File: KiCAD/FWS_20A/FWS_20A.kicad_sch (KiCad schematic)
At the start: 14 parts, among them J1 sense, J2 pwr, Q2 BC846, U1 XMSM0L1306SRGER, U2 FDMS8333L, U3 FDMS8333L, U4 LM5109BSD, U6 L78L33_SO8

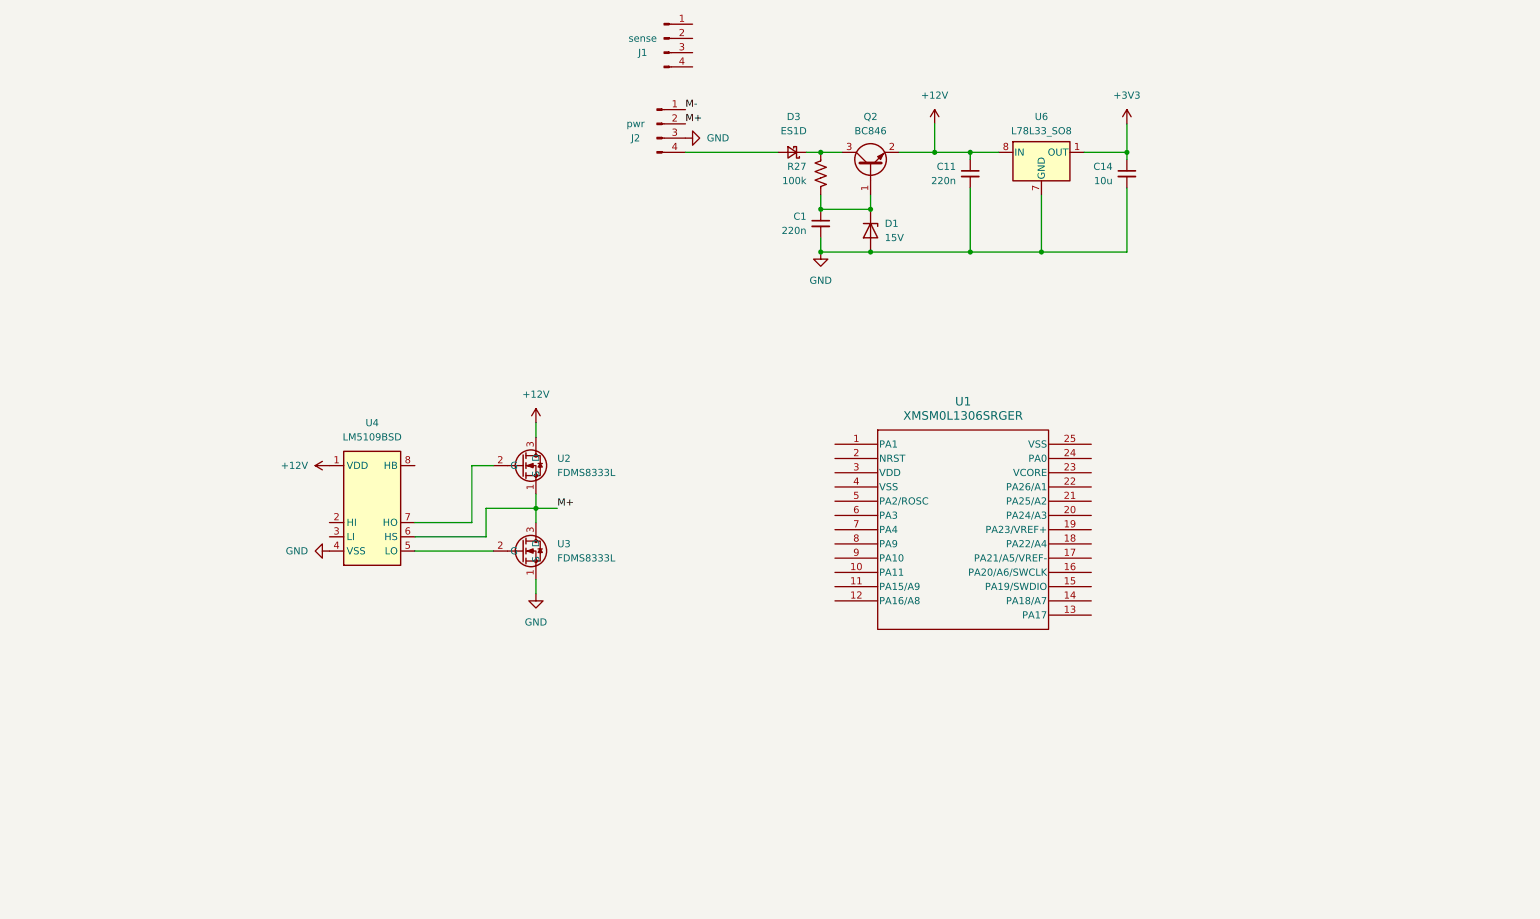
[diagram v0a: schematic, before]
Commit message: maybe schematic
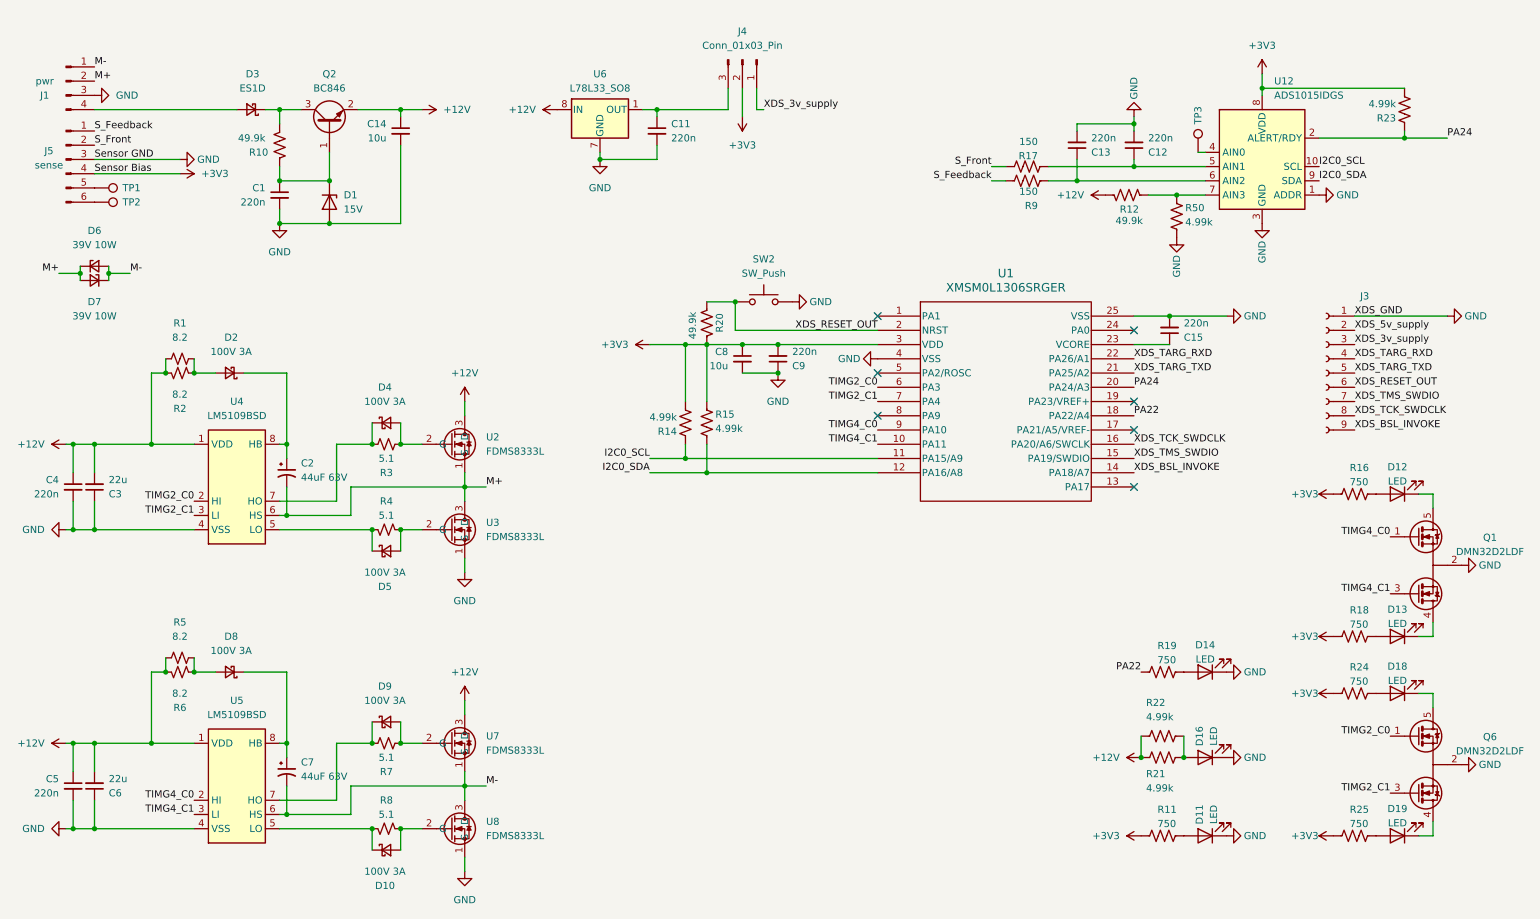
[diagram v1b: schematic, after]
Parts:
- removed J2: pwr, symbol Connector:Conn_01x04_Pin
- removed R27: 100k, Resistor_SMD:R_1206_3216Metric_Pad1.30x1.75mm_HandSolder, symbol Device:R_US
- added C12, C13, C15, C4, C5, C9: 220n, Capacitor_SMD:C_1206_3216Metric_Pad1.33x1.80mm_HandSolder, symbol Device:C_Small
- added C2, C7: 44uF 63V, Capacitor_THT:C_Radial_D6.3mm_H11.0mm_P2.50mm, symbol Device:C_Polarized_Small_US
- added C3, C6: 22u, Capacitor_SMD:C_1206_3216Metric_Pad1.33x1.80mm_HandSolder, symbol Device:C_Small
- added C8: 10u, Capacitor_SMD:C_1206_3216Metric_Pad1.33x1.80mm_HandSolder, symbol Device:C_Small
- added D10, D2, D4, D5, D8, D9: 100V 3A, FWS_footprints:PMDE, symbol Device:D_Schottky_Small
- added D11, D12, D13, D14, D16, D18, D19: LED, LED_SMD:LED_0603_1608Metric, symbol Device:LED
- added D6, D7: 39V 10W, Diode_SMD:D_SMC_Handsoldering, symbol Device:D_Zener_Small
- added J3: Conn_01x09_Socket, Connector_PinHeader_2.54mm:PinHeader_1x09_P2.54mm_Vertical, symbol Connector:Conn_01x09_Socket
- added J4: Conn_01x03_Pin, Connector_PinHeader_2.54mm:PinHeader_1x03_P2.54mm_Vertical, symbol Connector:Conn_01x03_Pin
- added J5: sense, Connector_Molex:Molex_Micro-Fit_3.0_43045-0600_2x03_P3.00mm_Horizontal, symbol Connector:Conn_01x06_Pin
- added Q1, Q6: DMN32D2LDF, Package_TO_SOT_SMD:SOT-353_SC-70-5, symbol Transistor_FET:DMN32D2LDF
- added R1, R2, R5, R6: 8.2, Resistor_SMD:R_2816_7142Metric_Pad3.20x4.45mm_HandSolder, symbol Device:R_Small_US
- added R10, R12, R20: 49.9k, Resistor_SMD:R_1206_3216Metric_Pad1.30x1.75mm_HandSolder, symbol Device:R_US
- added R11, R16, R18, R19, R24, R25: 750, Resistor_SMD:R_1206_3216Metric_Pad1.30x1.75mm_HandSolder, symbol Device:R_US
- added R14, R15, R21, R22, R23, R50: 4.99k, Resistor_SMD:R_1206_3216Metric_Pad1.30x1.75mm_HandSolder, symbol Device:R_US
- added R17, R9: 150, Resistor_SMD:R_1206_3216Metric_Pad1.30x1.75mm_HandSolder, symbol Device:R_US
- added R3, R4, R7, R8: 5.1, Resistor_SMD:R_2512_6332Metric_Pad1.40x3.35mm_HandSolder, symbol Device:R_Small_US
- added SW2: SW_Push, Button_Switch_SMD:SW_SPST_PTS645Sx43SMTR92, symbol Switch:SW_Push
- added TP1, TP2, TP3: TestPoint, TestPoint:TestPoint_Loop_D2.50mm_Drill1.0mm_LowProfile, symbol Connector:TestPoint
- added U12: ADS1015IDGS, Package_SO:TSSOP-10_3x3mm_P0.5mm, symbol Analog_ADC:ADS1015IDGS
- added U5: LM5109BSD, Package_SON:WSON-8-1EP_4x4mm_P0.8mm_EP2.6x3mm, symbol Driver_FET:LM5109BSD
- added U7, U8: FDMS8333L, FWS_footprints:Power 56, symbol FWS_symbols:FDMS8333L
- J1: value sense -> pwr; footprint (none) -> Connector_Wago:Wago_734-134_1x04_P3.50mm_Vertical
- U1: mouser (none) -> https://www.mouser.com/ProductDetail/Texas-Instruments/MSPM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
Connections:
- net +12V: now also C14.1, C3.2, C4.1, C5.1, C6.2, R1.2, R12.2, R2.2, R21.2, R22.1, R5.2, R6.2, U5.1 (VDD), U7.3 (D); no longer C11.1
- net +3V3: now also U1.3 (VDD), C8.1, C9.2, J4.2 (Pin_2), J5.4 (Pin_4), R11.2, R14.2, R15.1, R16.2, R18.2, R20.1, R23.2, R24.2, R25.2, U12.8 (VDD); no longer C14.1, U6.1 (OUT)
- net GND: now also J1.3 (Pin_3), U1.25 (VSS), U1.4 (VSS), C12.2, C13.2, C15.2, C3.1, C4.2, C5.2, C6.1, C8.2, C9.1, D11.1 (K), D14.1 (K), D16.1 (K), J3.1 (Pin_1), J5.3 (Pin_3), Q1.2 (S), Q6.2 (S), R50.2, SW2.2, U12.1 (ADDR), U12.3 (GND), U5.4 (VSS), U5.9 (VSS), U8.1 (S)
- net M+: now also J1.2 (Pin_2), C2.2, D6.1 (K), D7.2 (A)
- net M-: now also J1.1 (Pin_1), C7.2, D6.2 (A), D7.1 (K), U5.6 (HS), U7.1 (S), U8.3 (D)
- net at C1.1, D1.1 (K), Q2.1 (B): now also R10.1
- net at D3.1 (K), Q2.3 (C): now also R10.2
- net at D3.2 (A): now also J1.4 (Pin_4)
- net at U2.2 (G): now also D4.2 (A), R3.2; no longer U4.7 (HO)
- net TIMG4_C1: now reaches U1.10 (PA11)
- net TIMG4_C1: now also Q1.3 (G2), U5.3 (LI)
- net I2C0_SCL: now reaches U1.11 (PA15/A9)
- net I2C0_SCL: now also R14.1, U12.10 (SCL)
- net I2C0_SDA: now reaches U1.12 (PA16/A8)
- net I2C0_SDA: now also R15.2, U12.9 (SDA)
- net XDS_BSL_INVOKE: now reaches U1.14 (PA18/A7)
- net XDS_BSL_INVOKE: now also J3.9 (Pin_9)
- net XDS_TMS_SWDIO: now reaches U1.15 (PA19/SWDIO)
- net XDS_TMS_SWDIO: now also J3.7 (Pin_7)
- net XDS_TCK_SWDCLK: now reaches U1.16 (PA20/A6/SWCLK)
- net XDS_TCK_SWDCLK: now also J3.8 (Pin_8)
- net PA22: now reaches U1.18 (PA22/A4)
- net PA22: now also R19.2
- net XDS_RESET_OUT: now reaches U1.2 (NRST)
- net XDS_RESET_OUT: now also J3.6 (Pin_6), R20.2, SW2.1
- net PA24: now reaches U1.20 (PA24/A3)
- net PA24: now also R23.1, U12.2 (ALERT/RDY)
- net XDS_TARG_TXD: now reaches U1.21 (PA25/A2)
- net XDS_TARG_TXD: now also J3.5 (Pin_5)
- net XDS_TARG_RXD: now reaches U1.22 (PA26/A1)
- net XDS_TARG_RXD: now also J3.4 (Pin_4)
- net at U1.23 (VCORE): now also C15.1
- net TIMG2_C0: now reaches U1.6 (PA3)
- net TIMG2_C0: now also U4.2 (HI), Q6.1 (G1)
- net TIMG2_C1: now reaches U1.7 (PA4)
- net TIMG2_C1: now also U4.3 (LI), Q6.3 (G2)
- net TIMG4_C0: now reaches U1.9 (PA10)
- net TIMG4_C0: now also Q1.1 (G1), U5.2 (HI)
- net at U4.5 (LO): now also D5.1 (K), R4.1; no longer U3.2 (G)
- net at U4.8 (HB): now also C2.1, D2.1 (K)
- new net: D19.2 (A), R25.1
- new net: TP3.1, U12.4 (AIN0)
- new net: C12.1, R17.2, U12.5 (AIN1)
- new net: C13.1, R9.1, U12.6 (AIN2)
- new net: R12.1, R50.1, U12.7 (AIN3)
- new net: D19.1 (K), Q6.4 (D2)
- new net: D18.1 (K), Q6.5 (D1)
- new net: D2.2 (A), R1.1, R2.1
- new net: D11.2 (A), R11.1
- new net: D12.1 (K), Q1.5 (D1)
- new net: D12.2 (A), R16.1
- new net: D13.2 (A), R18.1
- new net: D9.2 (A), R7.2, U7.2 (G)
- new net: D14.2 (A), R19.1
- new net: D16.2 (A), R21.1, R22.2
- new net: D13.1 (K), Q1.4 (D2)
- new net: D10.1 (K), R8.1, U5.5 (LO)
- new net: D9.1 (K), R7.1, U5.7 (HO)
- new net: C7.1, D8.1 (K), U5.8 (HB)
- new net: C11.1, J4.3 (Pin_3), U6.1 (OUT)
- new net: J5.5 (Pin_5), TP1.1
- new net: D8.2 (A), R5.1, R6.1
- new net: D18.2 (A), R24.1
- new net: D4.1 (K), R3.1, U4.7 (HO)
- new net: J5.6 (Pin_6), TP2.1
- new net: D10.2 (A), R8.2, U8.2 (G)
- new net: D5.2 (A), R4.2, U3.2 (G)
- new net S_Feedback: J5.1 (Pin_1), R9.2
- new net S_Front: J5.2 (Pin_2), R17.1
- new net XDS_3v_supply: J3.3 (Pin_3), J4.1 (Pin_1)
- new net XDS_5v_supply: J3.2 (Pin_2)
- no-connect marks 0 -> 7
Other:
- moved on the sheet: C1, C11, C14, D1, D3, J1, Q2, U1, U2, U3, U4, U6
